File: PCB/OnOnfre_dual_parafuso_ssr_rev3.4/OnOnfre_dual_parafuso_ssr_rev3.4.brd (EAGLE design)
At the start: 44.4 x 47.7 mm, 24 parts, among them J3Y S8050, J7 8p, K1 OMRON-G3MB-202P-SSR2, K2 OMRON-G3MB-202P-SSR2, U2 esp12

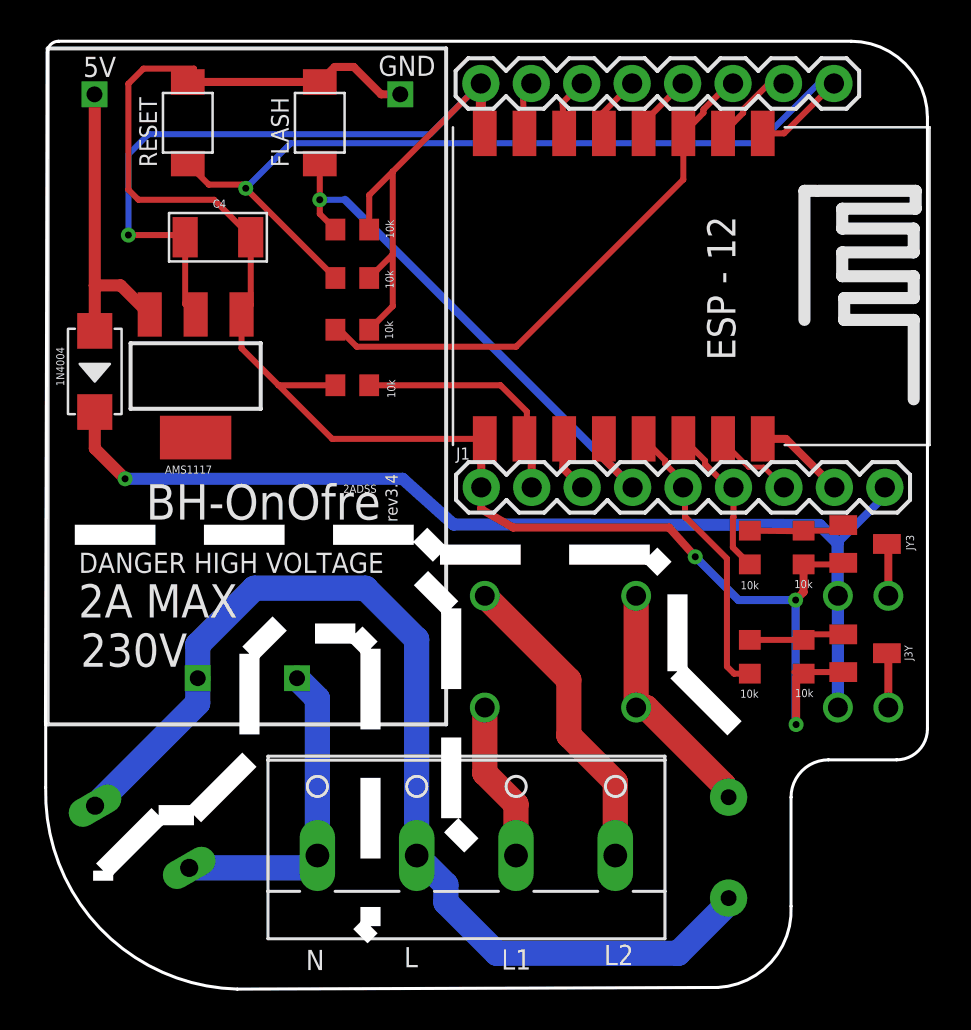
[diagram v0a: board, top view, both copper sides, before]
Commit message: Labels Fix
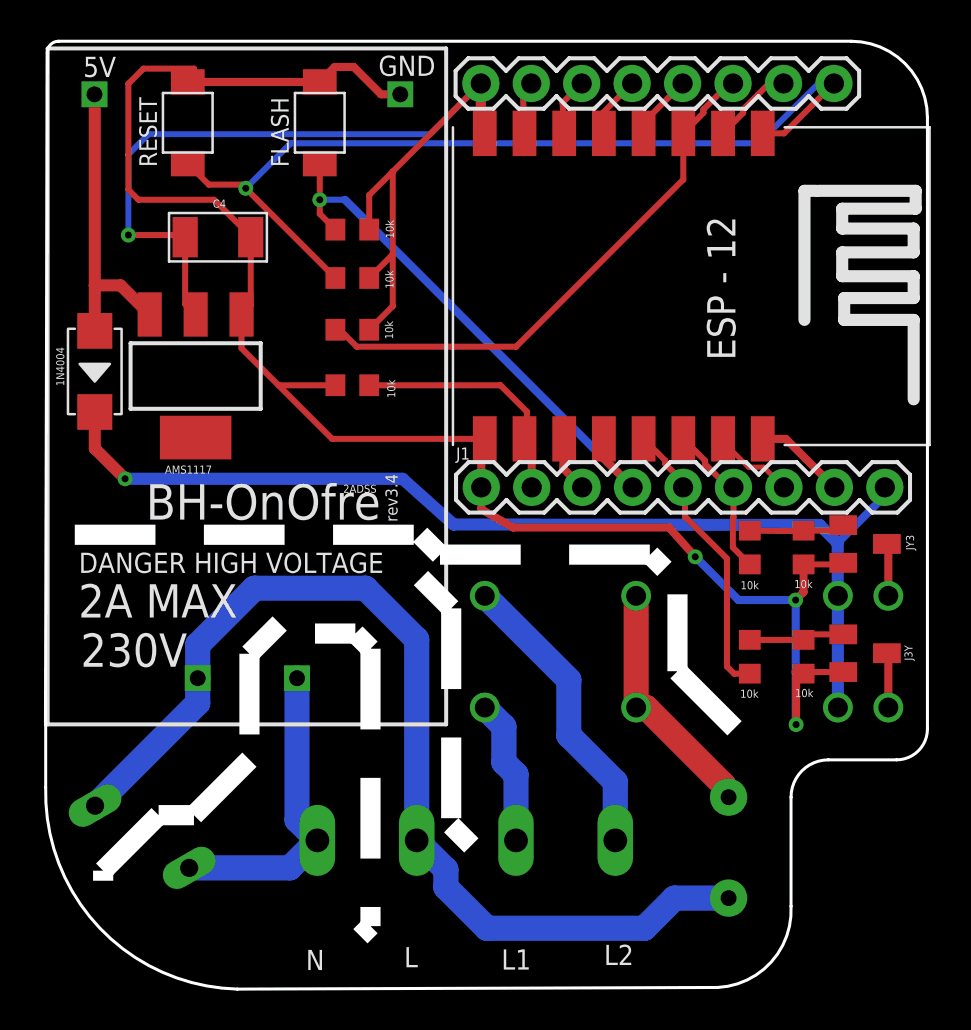
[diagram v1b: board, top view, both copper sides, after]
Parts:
- moved X1 1.78 mm to (21.6, 4.83), flipped to the bottom, turned to 180 degrees
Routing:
- net NEUTRAL_IN: track 54.0 -> 52.3 mm
- net NEUTRAL_TWO_OUT: track 15.8 -> 15.0 mm
- net NEUTRAL_ONE_OUT: track 8.10 -> 7.34 mm
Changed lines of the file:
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@@
 </element>
 <element name="J1" library="SparkFun-Connectors" library_urn="urn:adsk.eagle:library:513" package="1X09" package3d_urn="urn:adsk.eagle:package:38153/1" value="" x="22.342321875" y="23.872990625"/>
-<element name="X1" library="con-wago-500" library_urn="urn:adsk.eagle:library:195" package="W237-4" package3d_urn="urn:adsk.eagle:package:10695/1" value="" x="21.59" y="6.604" smashed="yes">
-<attribute name="MF" value="" x="21.59" y="6.604" size="1.778" layer="27" display="off"/>
-<attribute name="MPN" value="" x="21.59" y="6.604" size="1.778" layer="27" display="off"/>
-<attribute name="OC_FARNELL" value="unknown" x="21.59" y="6.604" size="1.778" layer="27" display="off"/>
-<attribute name="OC_NEWARK" value="unknown" x="21.59" y="6.604" size="1.778" layer="27" display="off"/>
-<attribute name="VALUE" x="13.9376" y="1.5748" size="1.27" layer="27" ratio="10"/>
+<element name="X1" library="con-wago-500" library_urn="urn:adsk.eagle:library:195" package="W237-4" package3d_urn="urn:adsk.eagle:package:10695/1" value="" x="21.59" y="4.826" smashed="yes" rot="MR180">
+<attribute name="MF" value="" x="21.59" y="4.826" size="1.778" layer="28" rot="MR180" display="off"/>
+<attribute name="MPN" value="" x="21.59" y="4.826" size="1.778" layer="28" rot="MR180" display="off"/>
+<attribute name="OC_FARNELL" value="unknown" x="21.59" y="4.826" size="1.778" layer="28" rot="MR180" display="off"/>
+<attribute name="OC_NEWARK" value="unknown" x="21.59" y="4.826" size="1.778" layer="28" rot="MR180" display="off"/>
+<attribute name="VALUE" x="13.9376" y="9.8552" size="1.27" layer="28" ratio="10" rot="MR180"/>
 </element>
 </elements>
@@
 <wire x1="10.922" y1="18.796" x2="16.51" y2="18.796" width="1.27" layer="16"/>
 <contactref element="X1" pad="2"/>
-<wire x1="19.09" y1="5.334" x2="20.55965" y2="3.86435" width="1.27" layer="16"/>
-<wire x1="20.55965" y1="3.86435" x2="20.55965" y2="2.976325" width="1.27" layer="16"/>
-<wire x1="20.55965" y1="2.976325" x2="23.125409375" y2="0.410565625" width="1.27" layer="16"/>
-<wire x1="23.125409375" y1="0.410565625" x2="32.25746875" y2="0.410565625" width="1.27" layer="16"/>
-<wire x1="32.25746875" y1="0.410565625" x2="34.79509375" y2="2.948190625" width="1.27" layer="16"/>
-<wire x1="34.79509375" y1="2.948190625" x2="34.79509375" y2="3.19045625" width="1.27" layer="16"/>
-<wire x1="19.09" y1="16.216" x2="19.09" y2="5.334" width="1.27" layer="16"/>
-<wire x1="16.51" y1="18.796" x2="19.09" y2="16.216" width="1.27" layer="16"/>
 <wire x1="2.8940875" y1="7.841953125" x2="8.064703125" y2="13.01256875" width="1.27" layer="16"/>
 <wire x1="8.064703125" y1="13.01256875" x2="8.064703125" y2="14.26316875" width="1.27" layer="16"/>
+<wire x1="16.51" y1="18.796" x2="19.09" y2="16.216" width="1.27" layer="16"/>
+<wire x1="19.09" y1="16.216" x2="19.09" y2="6.096" width="1.27" layer="16"/>
+<wire x1="34.79509375" y1="3.19045625" x2="32.07248125" y2="3.19045625" width="1.27" layer="16"/>
+<wire x1="32.07248125" y1="3.19045625" x2="30.552325" y2="1.6703" width="1.27" layer="16"/>
+<wire x1="22.627675" y1="1.6703" x2="20.55965" y2="3.738325" width="1.27" layer="16"/>
+<wire x1="20.55965" y1="3.738325" x2="20.55965" y2="4.62635" width="1.27" layer="16"/>
+<wire x1="20.55965" y1="4.62635" x2="19.09" y2="6.096" width="1.27" layer="16"/>
+<wire x1="30.552325" y1="1.6703" x2="22.627675" y2="1.6703" width="1.27" layer="16"/>
 </signal>
 <signal name="NEUTRAL_TWO_OUT" class="1">
 <contactref element="K2" pad="1"/>
-<wire x1="22.519509375" y1="18.410478125" x2="26.7505125" y2="14.179475" width="1.27" layer="1"/>
-<wire x1="26.7505125" y1="14.179475" x2="26.7505125" y2="11.3822" width="1.27" layer="1"/>
 <contactref element="X1" pad="4"/>
-<wire x1="29.09" y1="9.0427125" x2="29.09" y2="5.334" width="1.27" layer="1"/>
-<wire x1="26.7505125" y1="11.3822" x2="29.09" y2="9.0427125" width="1.27" layer="1"/>
+<wire x1="22.519509375" y1="18.410478125" x2="26.7505125" y2="14.179475" width="1.27" layer="16"/>
+<wire x1="26.7505125" y1="14.179475" x2="26.7505125" y2="11.3822" width="1.27" layer="16"/>
+<wire x1="29.09" y1="9.0427125" x2="29.09" y2="6.096" width="1.27" layer="16"/>
+<wire x1="26.7505125" y1="11.3822" x2="29.09" y2="9.0427125" width="1.27" layer="16"/>
 </signal>
 <signal name="NEUTRAL_ONE_OUT" class="1">
 <contactref element="K1" pad="1"/>
 <contactref element="X1" pad="3"/>
-<wire x1="22.5195125" y1="12.785975" x2="22.5195125" y2="9.4844875" width="1.27" layer="1"/>
-<wire x1="24.09" y1="7.914" x2="24.09" y2="5.334" width="1.27" layer="1"/>
-<wire x1="22.5195125" y1="9.4844875" x2="24.09" y2="7.914" width="1.27" layer="1"/>
+<wire x1="22.5195125" y1="12.785975" x2="23.4805125" y2="11.824975" width="1.27" layer="16"/>
+<wire x1="23.4805125" y1="11.824975" x2="23.4805125" y2="10.02771875" width="1.27" layer="16"/>
+<wire x1="23.4805125" y1="10.02771875" x2="24.09" y2="9.41823125" width="1.27" layer="16"/>
+<wire x1="24.09" y1="9.41823125" x2="24.09" y2="6.096" width="1.27" layer="16"/>
 </signal>
 <signal name="N$9">
@@
 <contactref element="R5" pad="1"/>
 <contactref element="X1" pad="1"/>
-<wire x1="14.09" y1="5.334" x2="13.46854375" y2="4.71254375" width="1.27" layer="16"/>
-<wire x1="13.46854375" y1="4.71254375" x2="7.633790625" y2="4.71254375" width="1.27" layer="16"/>
-<wire x1="14.09" y1="5.334" x2="14.09" y2="13.237871875" width="1.27" layer="16"/>
-<wire x1="14.09" y1="13.237871875" x2="13.064703125" y2="14.26316875" width="1.27" layer="16"/>
+<wire x1="13.064703125" y1="14.26316875" x2="13.064703125" y2="7.121296875" width="1.27" layer="16"/>
+<wire x1="13.064703125" y1="7.121296875" x2="14.09" y2="6.096" width="1.27" layer="16"/>
+<wire x1="14.09" y1="6.096" x2="12.70654375" y2="4.71254375" width="1.27" layer="16"/>
+<wire x1="12.70654375" y1="4.71254375" x2="7.633790625" y2="4.71254375" width="1.27" layer="16"/>
 </signal>
 </signals>
